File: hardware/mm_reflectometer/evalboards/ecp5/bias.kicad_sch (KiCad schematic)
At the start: 35 parts, among them J601 Conn_Coaxial, J602 Conn_Coaxial, U101 ECP5U_25_CABGA256, U603 ADS7868, U604 DAC7563SDSCR, U605 OPA2140, U606 TS5A23166

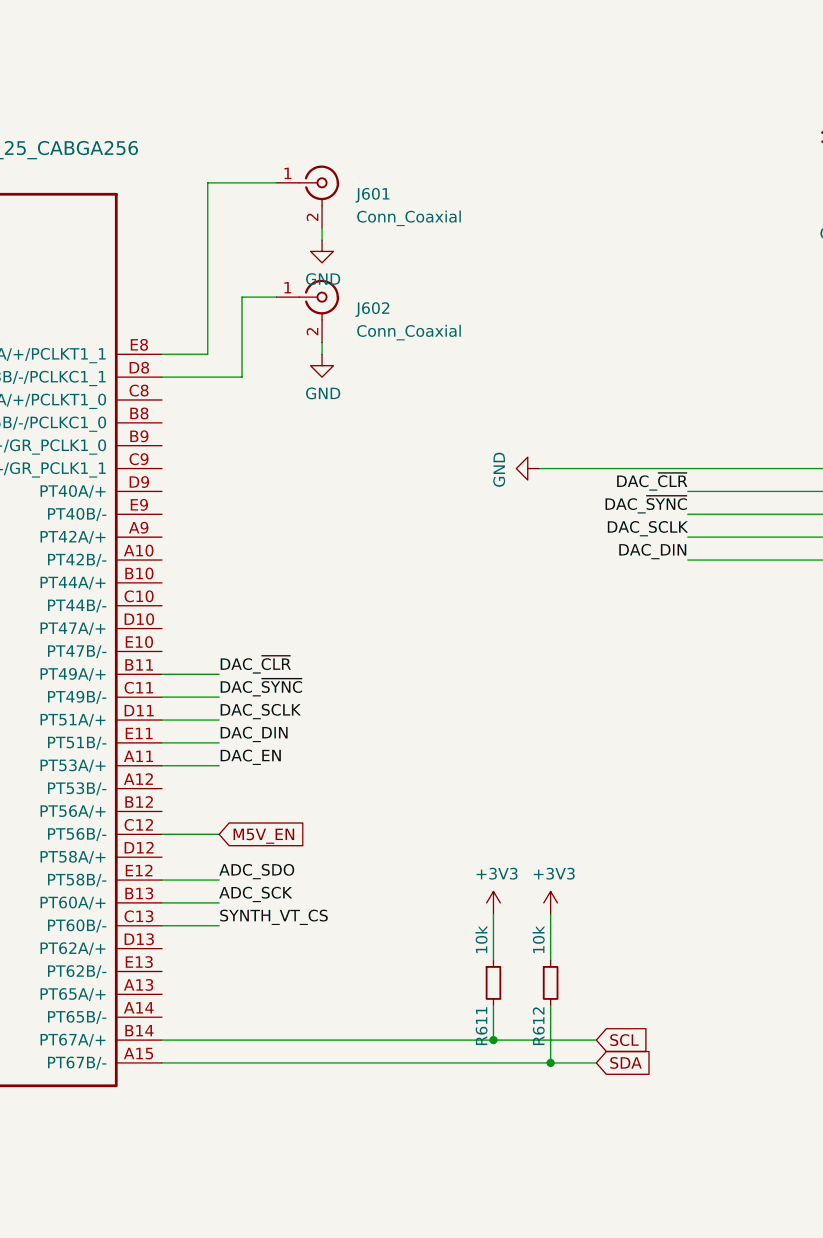
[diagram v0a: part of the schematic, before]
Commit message: routing on ecp5 eval board
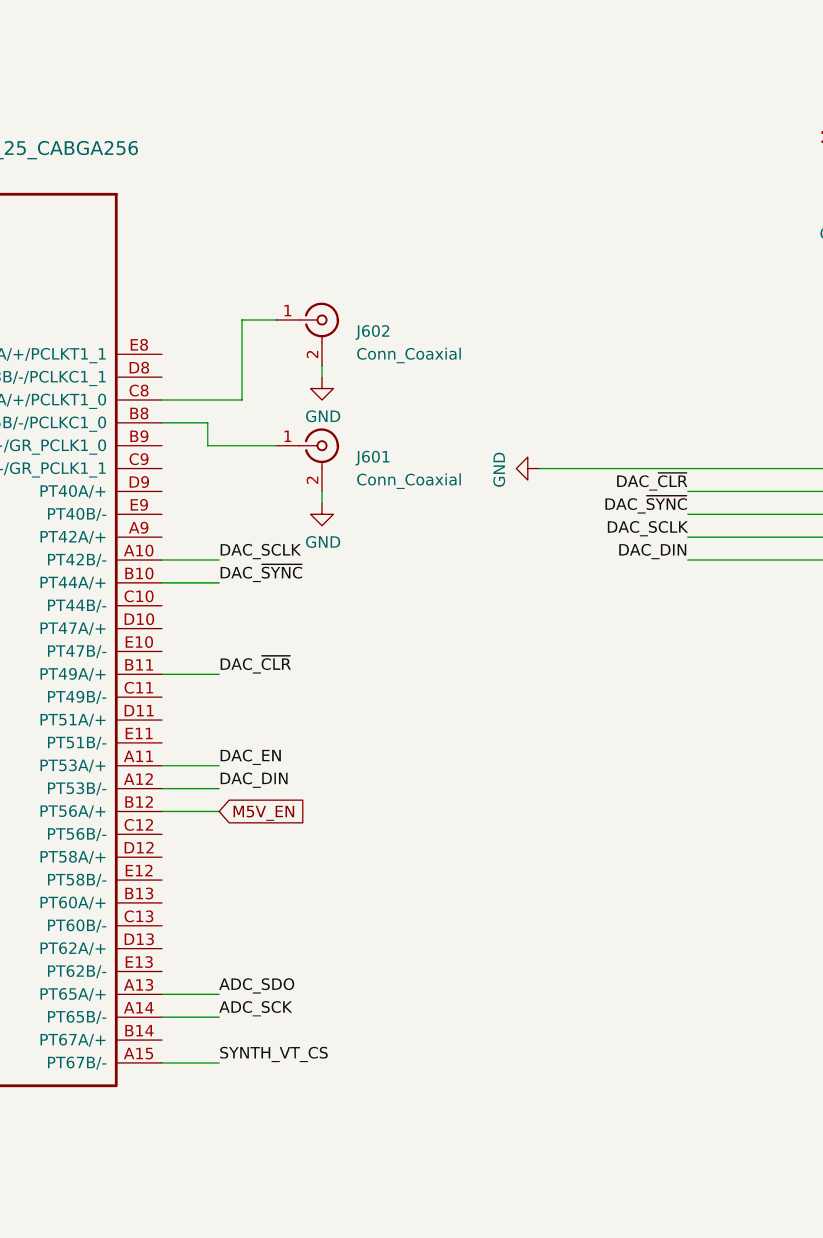
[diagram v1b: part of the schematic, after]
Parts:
- removed R611, R612: 10k, Resistor_SMD:R_0402_1005Metric, symbol Device:R_Small
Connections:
- net SDA is gone; now on net SYNTH_VT_CS: U101.A15 (PT67B/-)
- net ADC_SCK: now also U101.A14 (PT65B/-); no longer U101.B13 (PT60A/+)
- net ADC_SDO: now also U101.A13 (PT65A/+); no longer U101.E12 (PT58B/-)
- net DAC_DIN: now also U101.A12 (PT53B/-); no longer U101.E11 (PT51B/-)
- net DAC_SCLK: now also U101.A10 (PT42B/-); no longer U101.D11 (PT51A/+)
- net DAC_~SYNC: now also U101.B10 (PT44A/+); no longer U101.C11 (PT49B/-)
- net M5V_EN: now also U101.B12 (PT56A/+); no longer U101.C12 (PT56B/-)
- net SYNTH_VT_CS: no longer U101.C13 (PT60B/-)
- net at U101.B8 (PT35B/-/PCLKC1_0): now also J601.1 (In)
- net at U101.C8 (PT35A/+/PCLKT1_0): now also J602.1 (In)
- net at U101.D8 (PT33B/-/PCLKC1_1): no longer J602.1 (In)
- net at U101.E8 (PT33A/+/PCLKT1_1): no longer J601.1 (In)
- net SCL: no longer names the net of U101.B14 (PT67A/+)
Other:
- moved on the sheet: J601, J602
